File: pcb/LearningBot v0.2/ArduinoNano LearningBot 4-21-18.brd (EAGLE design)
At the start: 106.9 x 61.4 mm, 22 parts

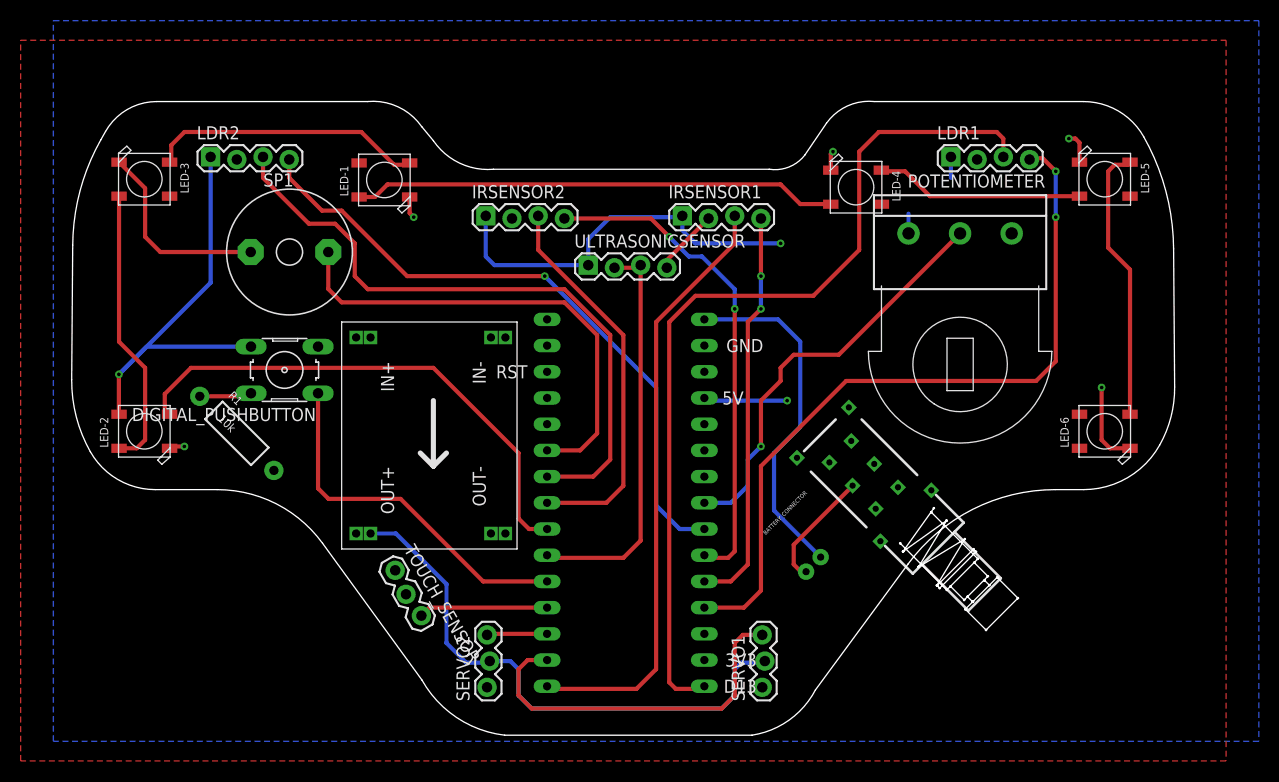
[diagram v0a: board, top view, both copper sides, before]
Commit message: Ready for inspection
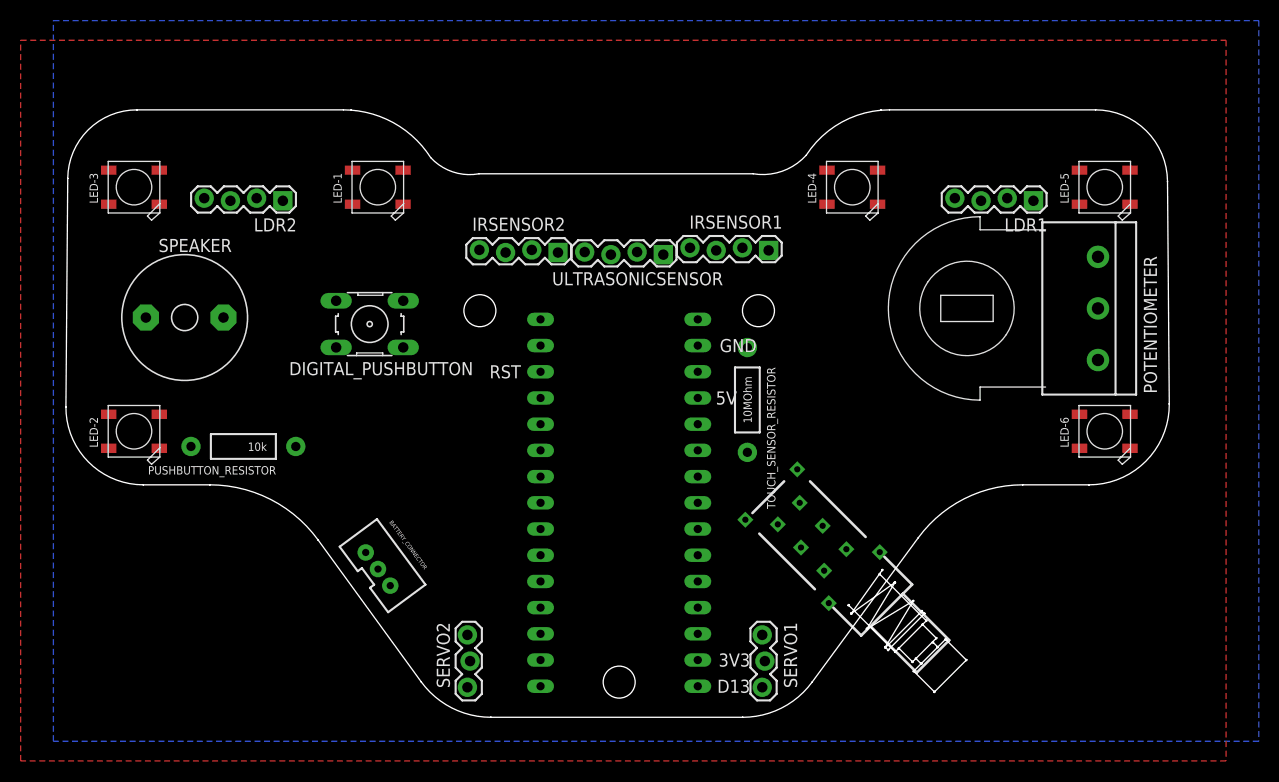
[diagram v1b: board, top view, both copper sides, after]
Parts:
- removed R1: 10k, SparkFun-Passives:AXIAL-0.4
- removed SP1: SPEAKER/AL60P, adafruit:AL60P
- removed TOUCH_SENSOR: (no value), SparkFun-Connectors:1X03_LOCK
- removed U$3: MP1584, MP1584-dc-brick:DC-BRICK
- added PUSHBUTTON_RESISTOR: 10k, SparkFun-Passives:AXIAL-0.4
- added SPEAKER: SPEAKER/AL60P, adafruit:AL60P
- added TOUCH_SENSOR_RESISTOR: 10MOhm, SparkFun-Passives:AXIAL-0.4
- BATTERY_CONNECTOR: device SparkFun-Connectors:JST-2-PTH-NS -> SparkFun-Connectors:JST-3-PTH-VERT
- moved BATTERY_CONNECTOR 41.8 mm to (34.4, 19.6), turned to 306.5 degrees
- moved POTENTIOMETER 15.2 mm to (103.8, 44.5), turned to 90 degrees
- moved DIGITAL_PUSHBUTTON 9.38 mm to (33.2, 43.0)
- moved LDR1 8.94 mm to (97.5, 55.1), turned to 180 degrees
- moved IRSENSOR1 8.92 mm to (71.9, 50.2), turned to 180 degrees
- moved LDR2 8.06 mm to (24.8, 55.1), turned to 180 degrees
- moved POWER_SWITCH 7.81 mm to (75.9, 22.2)
- moved IRSENSOR2 7.74 mm to (51.5, 50.0), turned to 180 degrees
- moved ULTRASONICSENSOR 7.39 mm to (61.7, 49.8), turned to 180 degrees
- moved SERVO2 1.91 mm to (42.8, 7.77)
- moved LED-3 1.27 mm to (10.4, 56.2), turned to 180 degrees
- moved LED-2 1.00 mm to (10.4, 32.6)
- moved LED-1 0.95 mm to (34.0, 56.2)
- moved LED-5 0.78 mm to (104.4, 56.2), turned to 180 degrees
- moved U$1 0.63 mm to (54.8, 34.5)
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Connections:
- removed net SERVO1_PIN: SERVO1.3, U$1.D11
- removed net TOUCH_SENSOR: TOUCH_SENSOR.3, U$1.D9
- removed net ULTRASONICSENSOR_PIN: U$1.D7, ULTRASONICSENSOR.2, ULTRASONICSENSOR.3
- new net CAP_TOUCH_RECEIVE_PIN: TOUCH_SENSOR_RESISTOR.P$1, U$1.A6
- new net CAP_TOUCH_SEND_PIN: TOUCH_SENSOR_RESISTOR.P$2, U$1.A5
- new net ECHO_PIN: U$1.D6, ULTRASONICSENSOR.3
- new net TRIG_PIN: U$1.D7, ULTRASONICSENSOR.2
- net GND: now also POWER_SWITCH.NO1, PUSHBUTTON_RESISTOR.P$2, SPEAKER.1; no longer POWER_SWITCH.NC1, R1.P$2, SP1.1, TOUCH_SENSOR.1, U$3.IN1-, U$3.IN2-, U$3.OUT1-, U$3.OUT2-
- net LED-1: now also U$1.D9; no longer U$1.D6
- net N$3: now also PUSHBUTTON_RESISTOR.P$1; no longer R1.P$1
- net N$9: now also BATTERY_CONNECTOR.3; no longer BATTERY_CONNECTOR.1
- net RAWIN: now also BATTERY_CONNECTOR.1; no longer BATTERY_CONNECTOR.2
- net SERVOVCC: no longer U$3.OUT1+, U$3.OUT2+
- net SPEAKERPIN: now also SPEAKER.2; no longer SP1.2
- net VCC: now also SERVO1.3, U$1.D11; no longer TOUCH_SENSOR.2, U$3.IN1+, U$3.IN2+
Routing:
- net VCC: track 92.9 -> 0.00 mm, vias 3 -> 0
- net LDR1_DO: track 86.3 -> 0.00 mm
- net LDR1_AO: track 72.6 -> 0.00 mm, vias 2 -> 0
- net LDR2_AO: track 62.8 -> 0.00 mm, vias 1 -> 0
- net LDR2_DO: track 62.7 -> 0.00 mm
- net IR_SENSOR1_DO: track 58.6 -> 0.00 mm
- net SERVOVCC: track 53.6 -> 0.00 mm
- net LED-1: track 50.5 -> 0.00 mm
- net IR_SENSOR2_AO: track 48.1 -> 0.00 mm, vias 2 -> 0
- net N$6: track 47.0 -> 0.00 mm
- net SPEAKERPIN: track 46.6 -> 0.00 mm
- net GND: track 42.3 -> 0.00 mm, vias 5 -> 0
- net POTPIN: track 40.4 -> 0.00 mm, vias 1 -> 0
- net ULTRASONICSENSOR_PIN: track 39.2 -> 0.00 mm
- net IR_SENSOR1_AO: track 39.0 -> 0.00 mm, vias 2 -> 0
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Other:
- board size 106.9 x 61.4 mm -> 106.9 x 58.9 mm
